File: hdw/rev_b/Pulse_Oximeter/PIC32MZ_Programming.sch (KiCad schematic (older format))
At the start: 10 parts, among them J1501 PICKIT4, Q1501 BSS214NW, SW1501 MRST

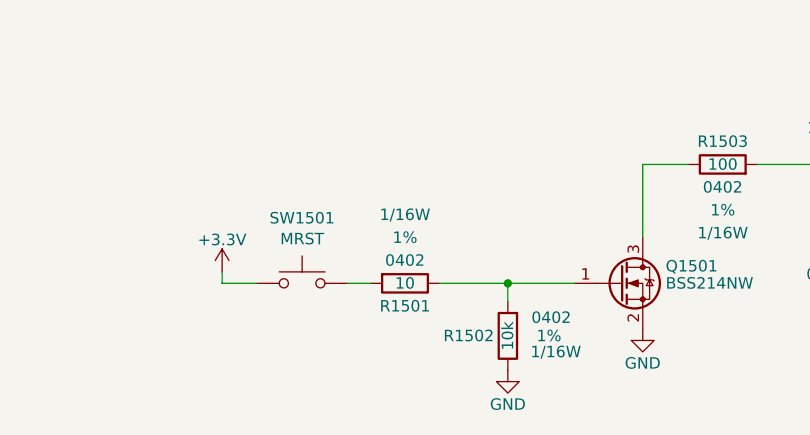
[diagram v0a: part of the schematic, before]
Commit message: few little tweaks
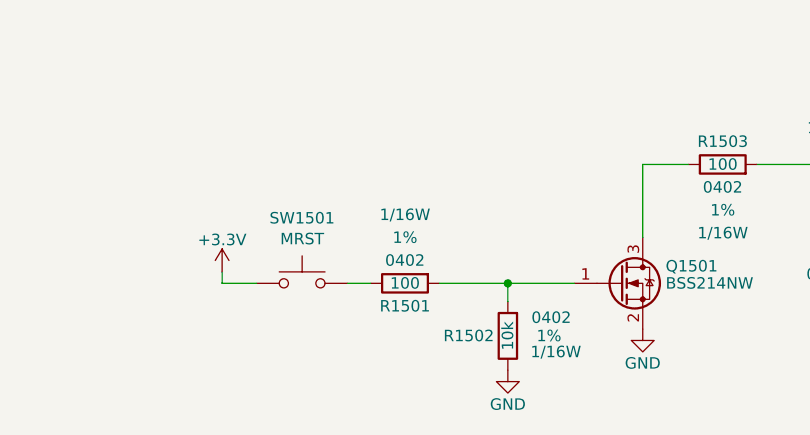
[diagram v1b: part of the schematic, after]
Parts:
- R1501: value 10 -> 100
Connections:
- net at SW1501.2: now also R1501.2; no longer R1501.1
- net at Q1501.1 (G), R1502.1: now also R1501.1; no longer R1501.2
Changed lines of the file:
@@
-$EndComp
-$Comp
-L Custom_Library:R_Custom R1501
-U 1 1 5BE087CB
-P 5470 2770
-F 0 "R1501" V 5370 2770 50  0000 C CNN
-F 1 "10" V 5470 2770 50  0000 C CNN
-F 2 "Resistors_SMD:R_0402" H 5470 2770 50  0001 C CNN
-F 3 "" H 5470 2770 50  0001 C CNN
-F 4 "0402" V 5570 2770 50  0000 C CNN "display_footprint"
-F 5 "1%" V 5670 2770 50  0000 C CNN "Tolerance"
-F 6 "1/16W" V 5770 2770 50  0000 C CNN "Wattage"
-F 7 "" H 5770 3170 60  0001 C CNN "Digi-Key PN"
-	1    5470 2770
-	0    -1   -1   0
 $EndComp
 $Comp
@@
 Wire Wire Line
 	1270 1990 2320 1990
+$Comp
+L Custom_Library:R_Custom R1501
+U 1 1 5FE81E3C
+P 5470 2770
+F 0 "R1501" V 5370 2770 50  0000 C CNN
+F 1 "100" V 5470 2770 50  0000 C CNN
+F 2 "Resistors_SMD:R_0402" H 5470 2770 50  0001 C CNN
+F 3 "" H 5470 2770 50  0001 C CNN
+F 4 "0402" V 5570 2770 50  0000 C CNN "display_footprint"
+F 5 "1%" V 5670 2770 50  0000 C CNN "Tolerance"
+F 6 "1/16W" V 5770 2770 50  0000 C CNN "Wattage"
+F 7 "" H 5770 3170 60  0001 C CNN "Digi-Key PN"
+	1    5470 2770
+	0    1    -1   0
+$EndComp
 $EndSCHEMATC
